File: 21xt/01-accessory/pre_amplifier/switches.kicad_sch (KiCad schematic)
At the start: 40 parts, among them IC13 MAX14774ATP+, IC14 MAX14774ATP+, IC15 MAX14774ATP+, IC16 MAX14774ATP+, IC17 MAX14774ATP+, IC18 MAX14774ATP+, IC19 MAX14774ATP+, IC20 MAX14774ATP+

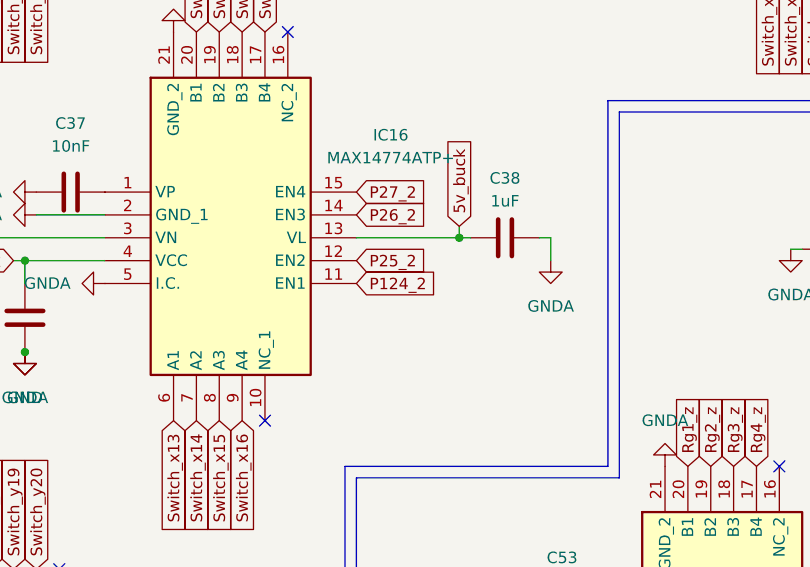
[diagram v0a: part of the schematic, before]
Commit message: fixing inputs
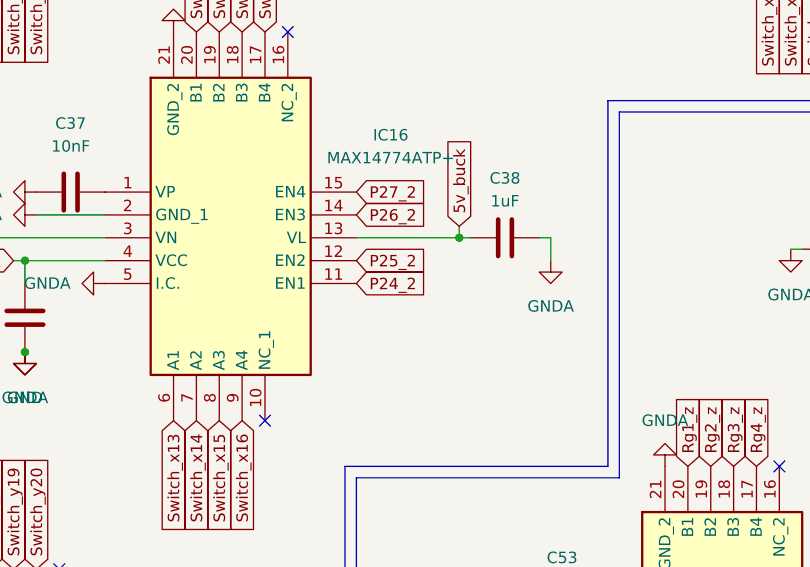
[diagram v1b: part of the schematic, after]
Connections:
- net P124_2 renamed P24_2
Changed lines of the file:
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@@
 		)
 	)
-	(global_label "P124_2"
+	(global_label "P24_2"
 		(shape input)
 		(at 95.25 105.41 0)
@@
 		)
 		(property "Intersheetrefs" "${INTERSHEET_REFS}"
-			(at 105.3108 105.41 0)
+			(at 104.1013 105.41 0)
 			(effects
 				(font
